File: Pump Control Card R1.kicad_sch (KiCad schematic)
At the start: 28 parts, among them J1 Conn_01x04, J2 Conn_01x04, J4 Conn_01x04, J5 Conn_01x04, J6 Conn_01x04, J7 Conn_01x04, J8 Conn_01x04, J9 Conn_01x04

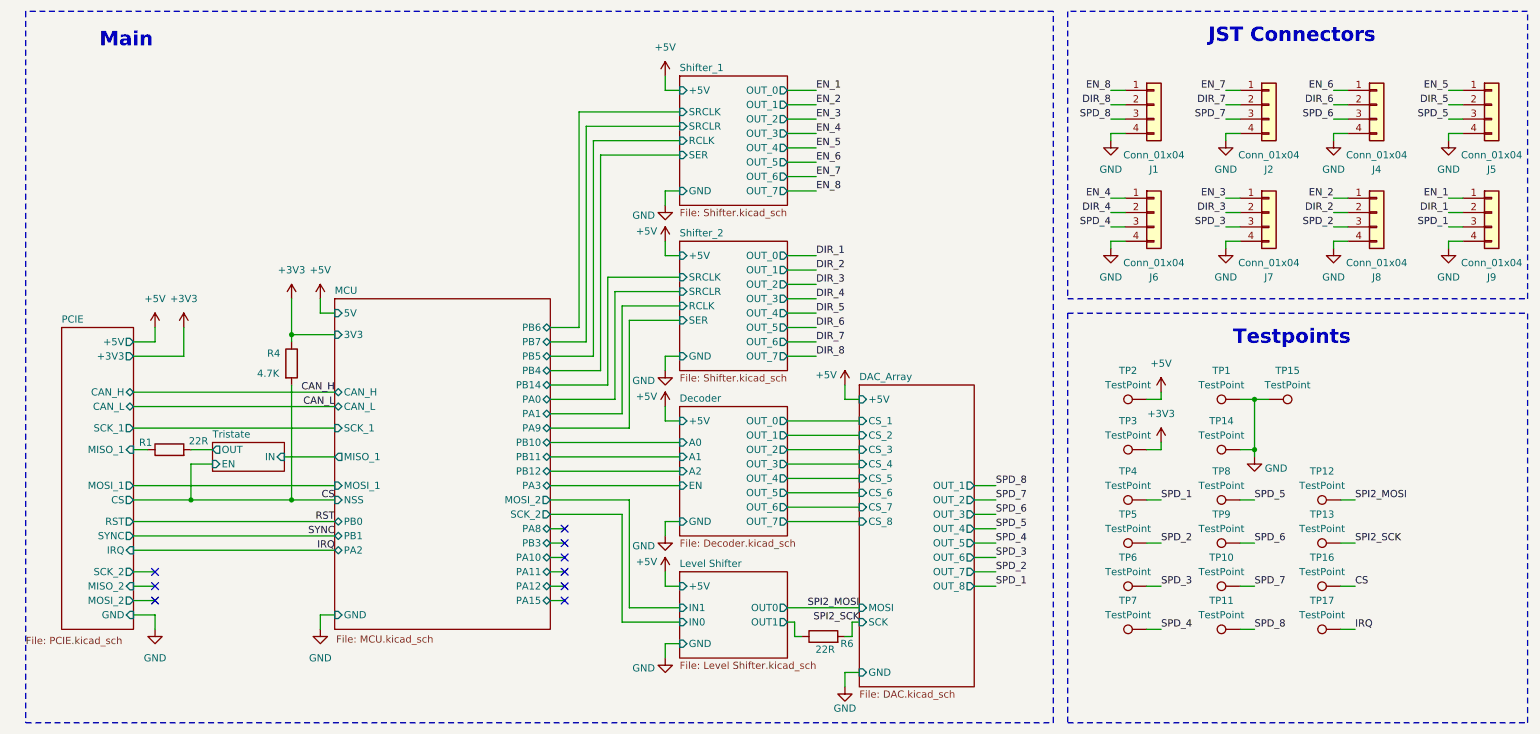
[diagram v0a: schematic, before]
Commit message: Updated
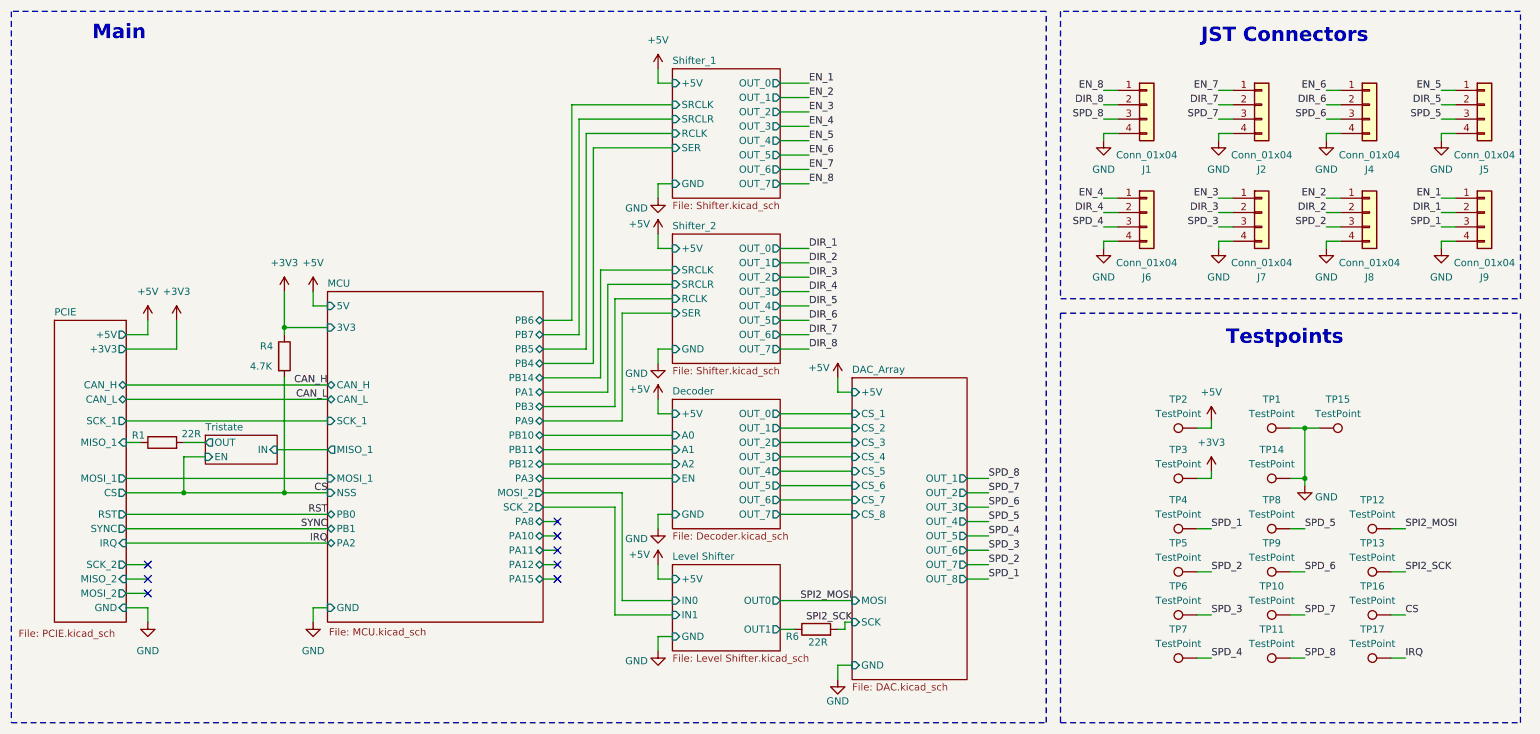
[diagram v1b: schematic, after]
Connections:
- no-connect marks 9 -> 8
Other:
- sheet MCU ports: added none; removed PA0
- moved on the sheet: J1, J2, J4, J5, J6, J7, J8, J9, R1, R4, R6, TP1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
